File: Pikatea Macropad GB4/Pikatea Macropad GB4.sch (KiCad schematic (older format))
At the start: 34 parts, among them J1 AVR-ISP-6, J2 USB_B_Mini, J6 Conn_01x06_Male, SW1 SW_DPST, SW2 Rotary_Encoder_Switch, U1 ATMEGA32U4-EP, X1 16MHz

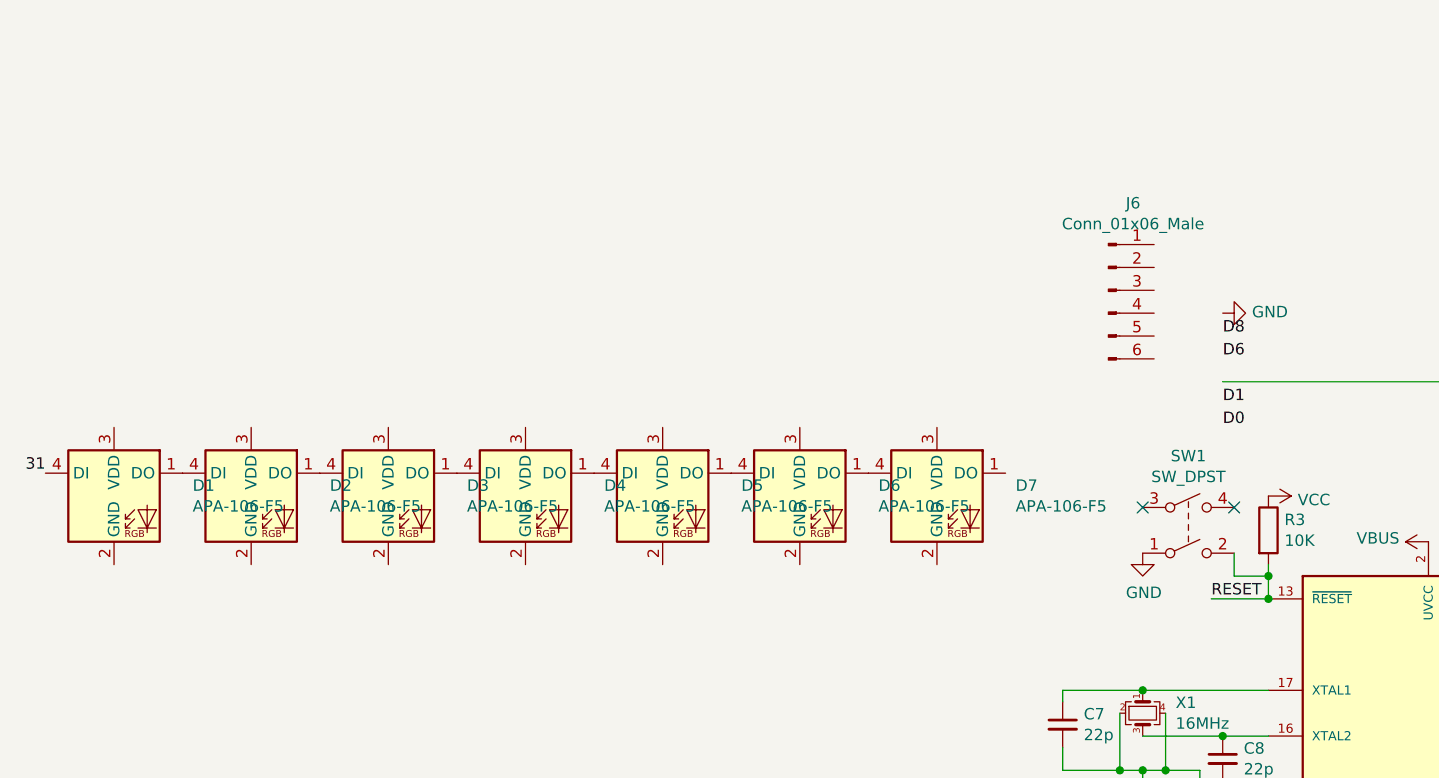
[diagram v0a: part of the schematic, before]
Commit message: Revision b of GB4
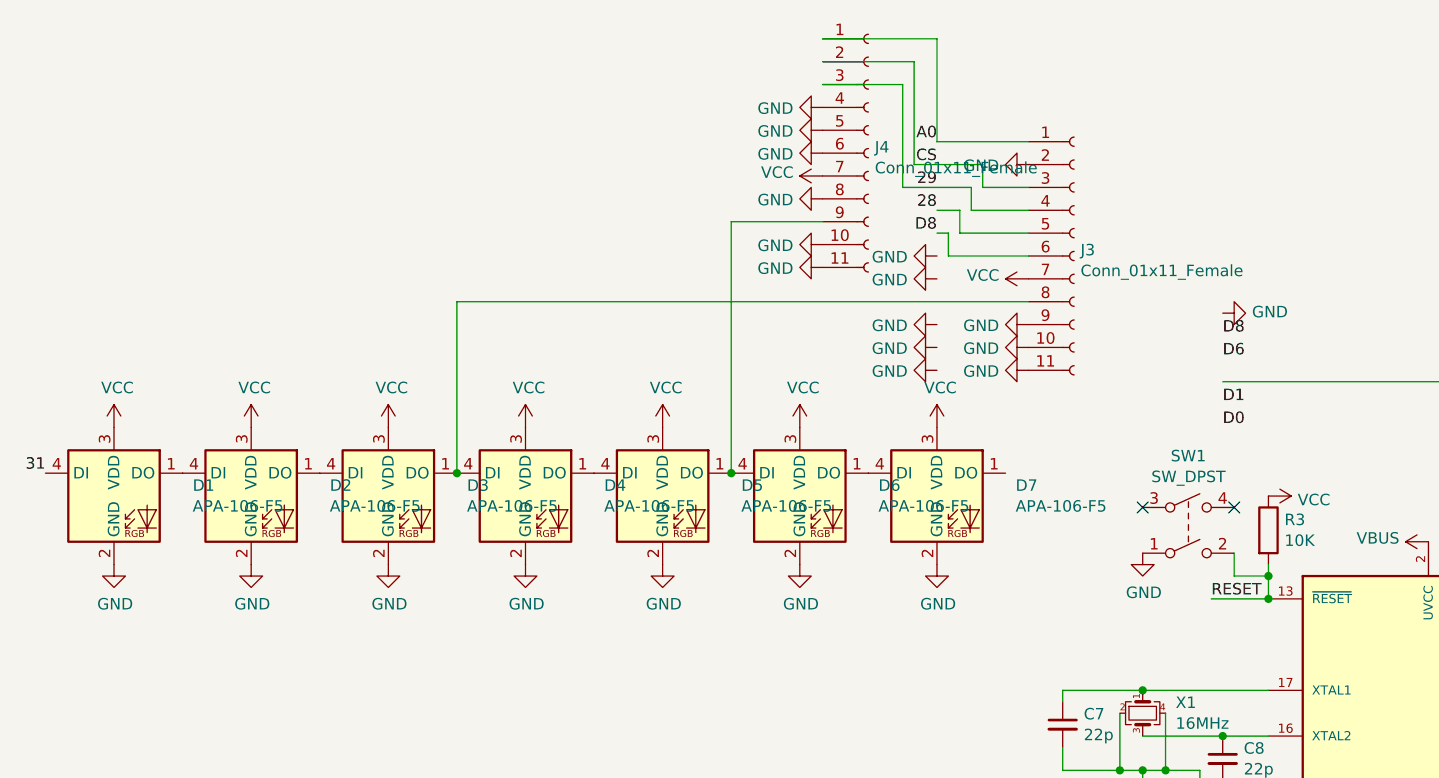
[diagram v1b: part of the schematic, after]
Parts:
- removed J6: Conn_01x06_Male, Pikatea Macropad Encoder Side Mount:Breakaway-Throughole, symbol Connector:Conn_01x06_Male
- added J3, J4: Conn_01x11_Female, Pikatea:Breakaway-Throughole-GB4, symbol Connector:Conn_01x11_Female
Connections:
- net 28: now also J3.5 (Pin_5)
- net 29: now also J3.4 (Pin_4), J4.3 (Pin_3)
- net A0: now also J3.1 (Pin_1), J4.1 (Pin_1)
- net CS: now also J3.3 (Pin_3), J4.2 (Pin_2)
- net D8: now also J3.6 (Pin_6)
- net GND: now also D1.2 (GND), D2.2 (GND), D3.2 (GND), D4.2 (GND), D5.2 (GND), D6.2 (GND), D7.2 (GND), J3.10 (Pin_10), J3.11 (Pin_11), J3.2 (Pin_2), J3.9 (Pin_9), J4.10 (Pin_10), J4.11 (Pin_11), J4.4 (Pin_4), J4.5 (Pin_5), J4.6 (Pin_6), J4.8 (Pin_8)
- net VBUS: now also D1.3 (VDD), D2.3 (VDD), D3.3 (VDD), D4.3 (VDD), D5.3 (VDD), D6.3 (VDD), D7.3 (VDD), J3.7 (Pin_7), J4.7 (Pin_7)
- net at D3.1 (DO), D4.4 (DI): now also J3.8 (Pin_8)
- net at D5.1 (DO), D6.4 (DI): now also J4.9 (Pin_9)
